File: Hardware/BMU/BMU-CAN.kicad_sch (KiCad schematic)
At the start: 6 parts, among them U5 MCP2562FDT-H_SN

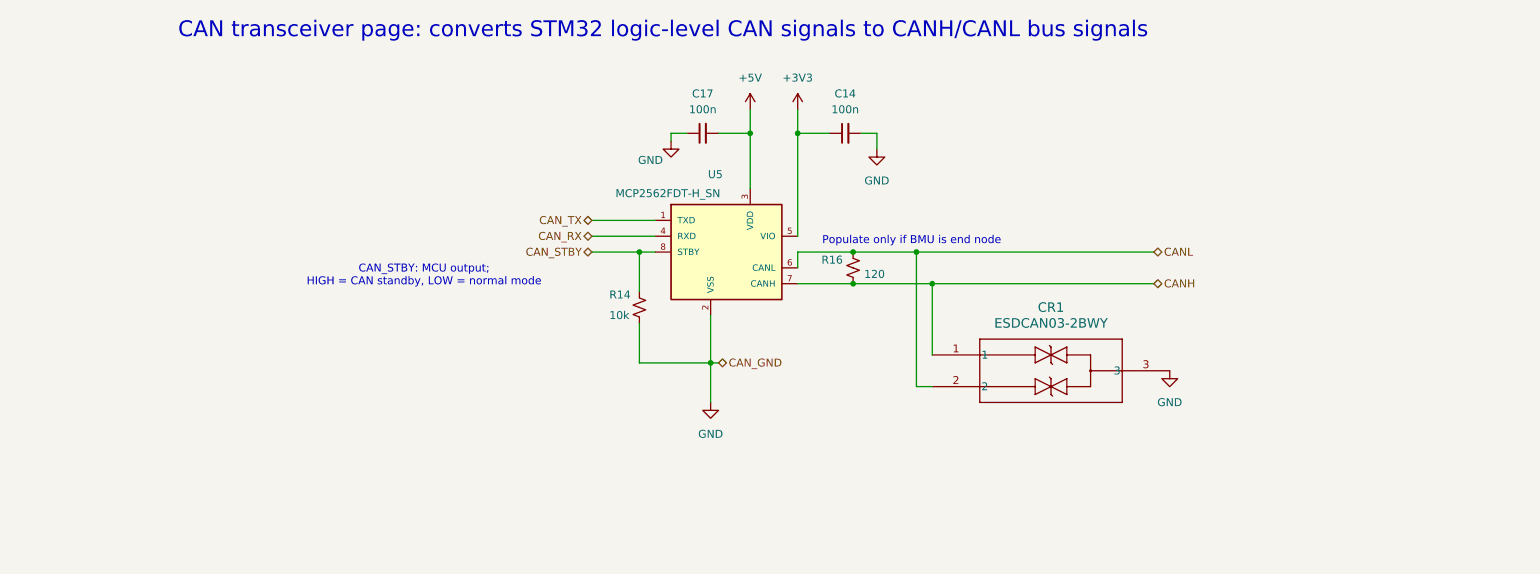
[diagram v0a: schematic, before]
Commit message: add footprint
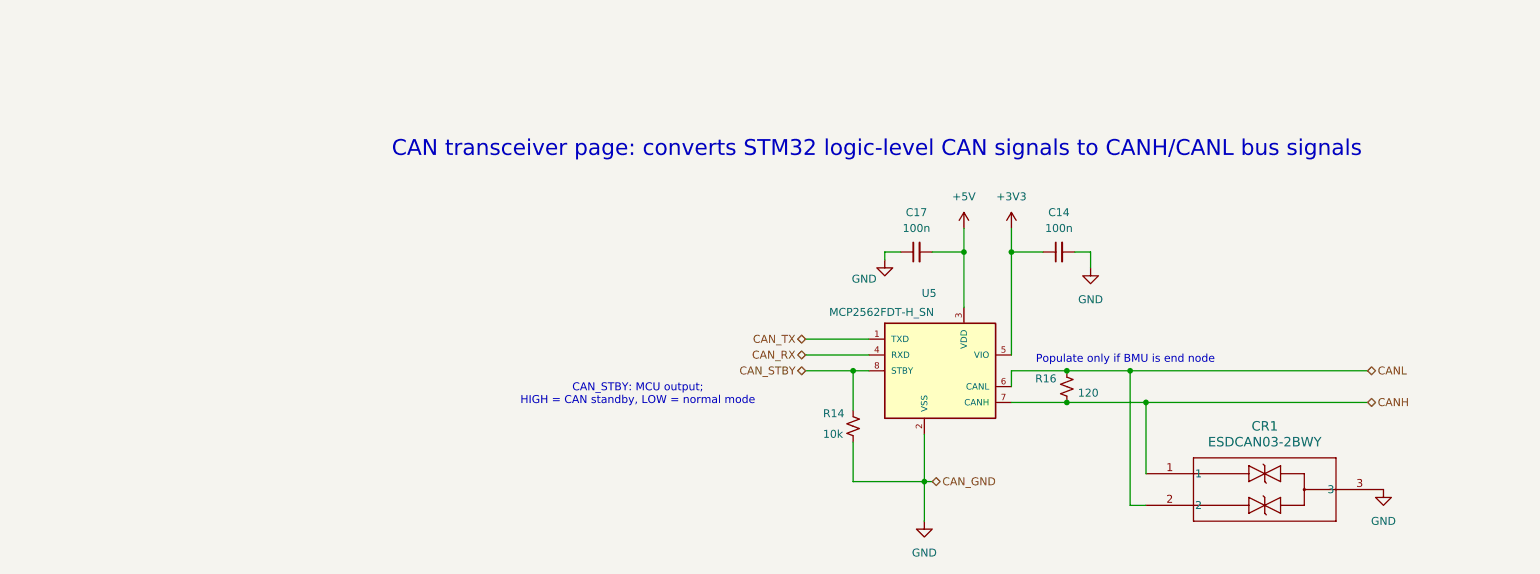
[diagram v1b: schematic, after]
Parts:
- C14, C17: footprint (none) -> Capacitor_SMD:C_0805_2012Metric
- CR1: footprint SOT323-3L_STM -> ESDCAN03-2BWY:SOT323-3L_STM
- R14, R16: footprint (none) -> Resistor_SMD:R_0805_2012Metric
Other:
- moved on the sheet: C14, C17, CR1, R14, R16, U5
